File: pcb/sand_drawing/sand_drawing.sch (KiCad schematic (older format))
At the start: 19 parts, among them J0 12V GND, J1 Stepper1, J2 Stepper2, J3 Opto 1, J4 Opto 2, J5 ESP POWER, J6 Unused Pins, U1 WeMos_D1_mini, U2 LD1117

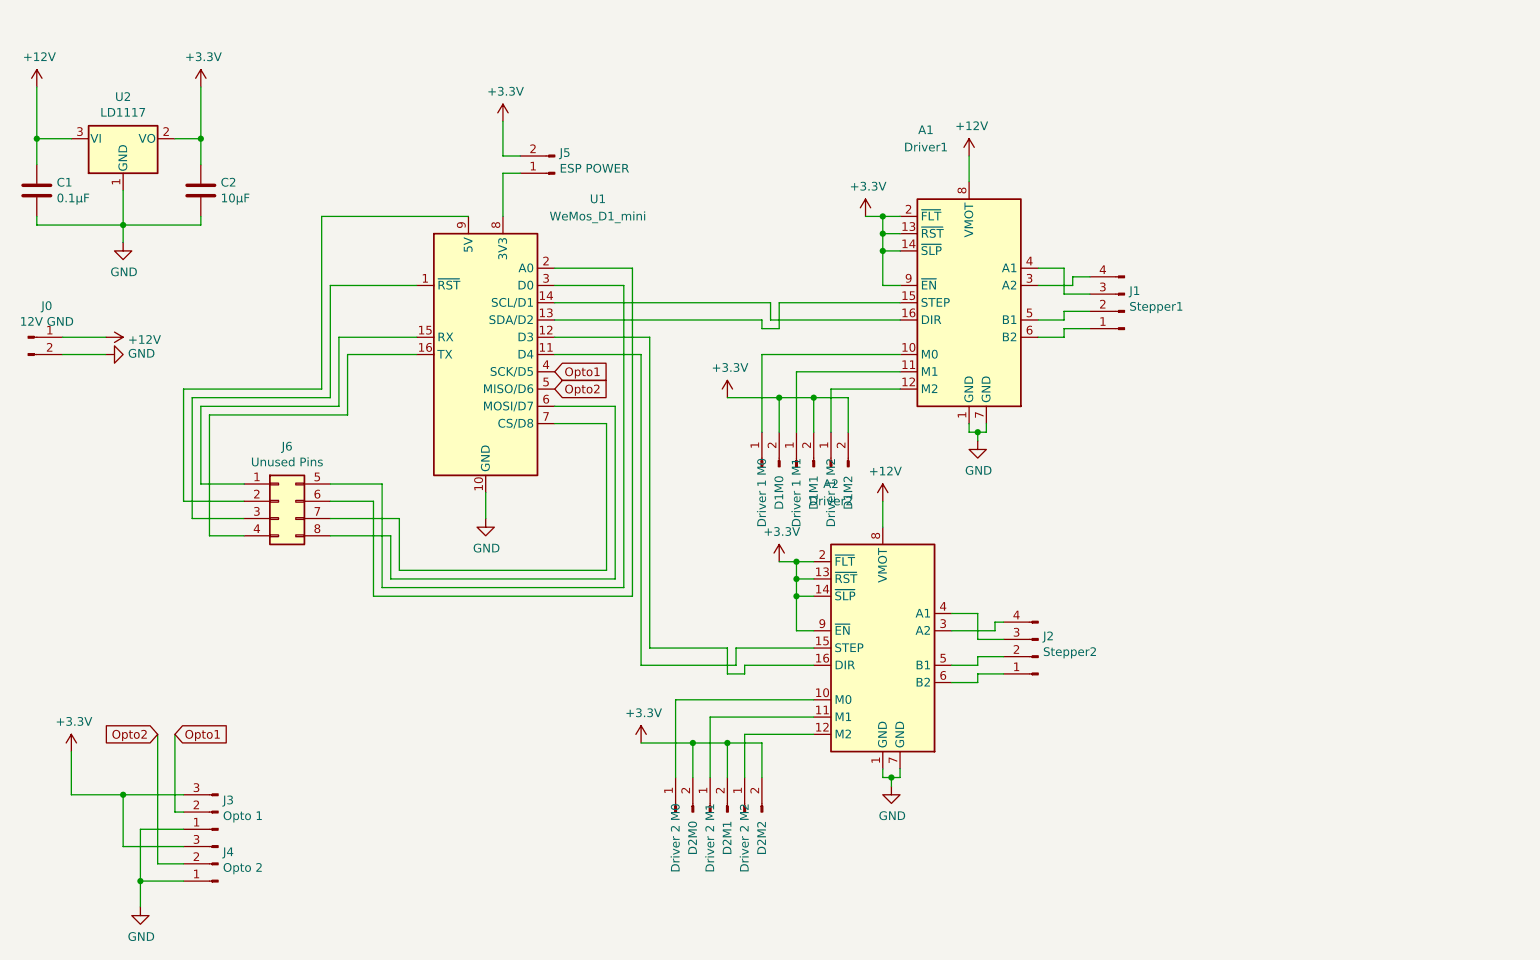
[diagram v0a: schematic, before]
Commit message: Tidy up schematic.
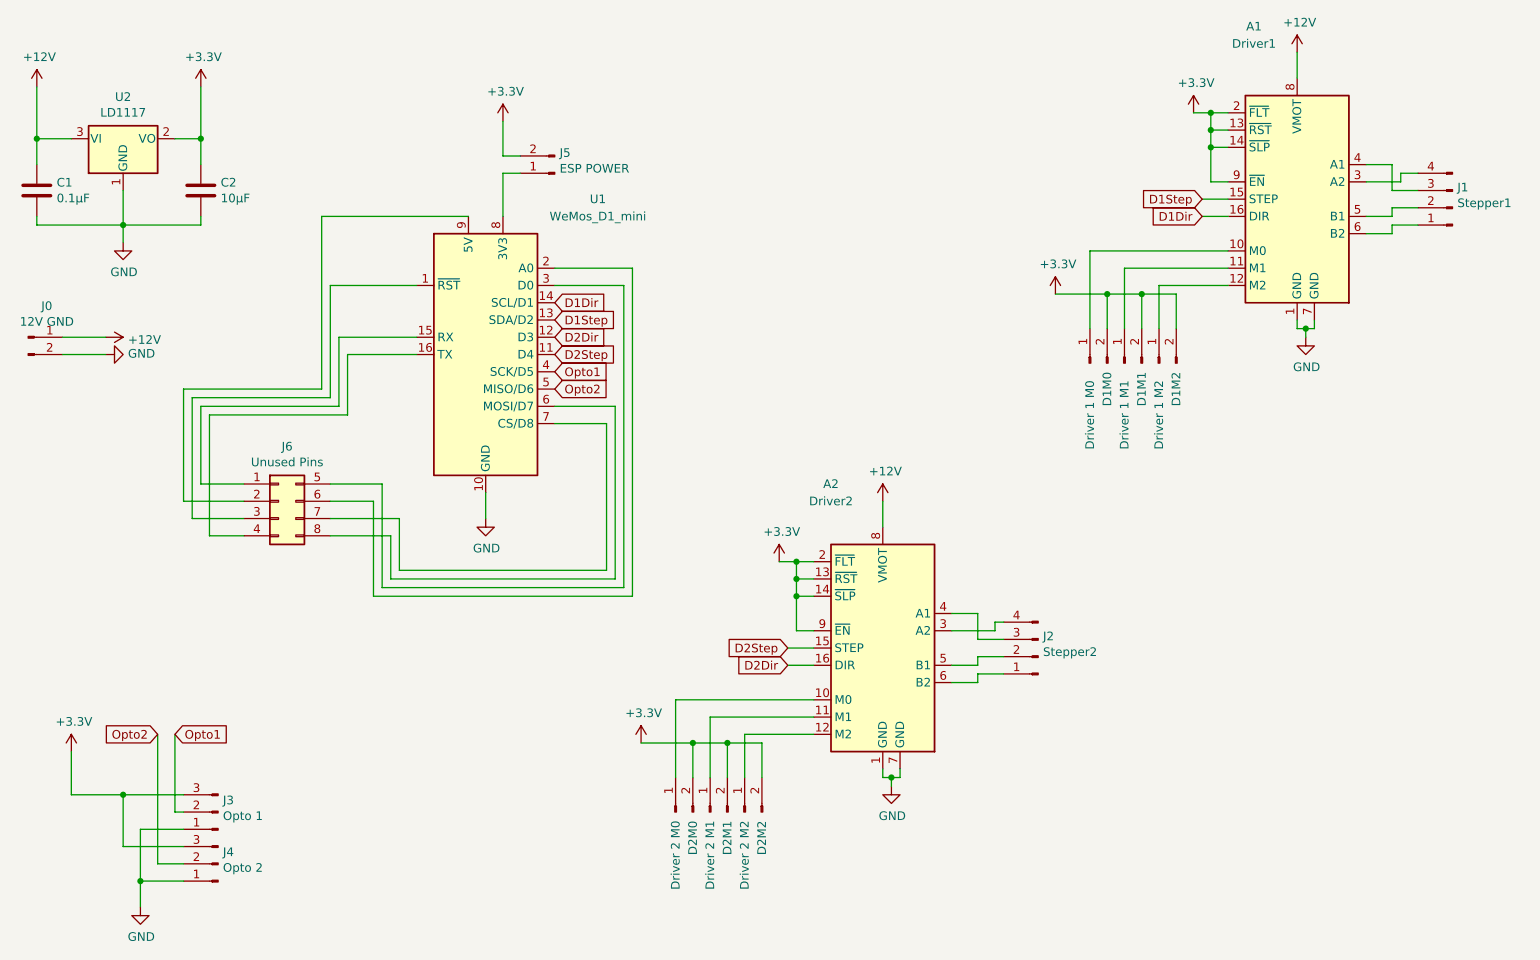
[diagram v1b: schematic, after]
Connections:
- net D2Step: now reaches A2.15 (STEP), U1.11 (D4)
- net D2Dir: now reaches A2.16 (DIR), U1.12 (D3)
- net D1Step: now reaches A1.15 (STEP), U1.13 (SDA/D2)
- net D1Dir: now reaches A1.16 (DIR), U1.14 (SCL/D1)
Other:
- moved on the sheet: A1, D1M0, D1M1, D1M2, J1
